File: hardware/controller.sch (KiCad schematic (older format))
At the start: 13 parts, among them U1 STM32F103C8Tx, Y1 16Mhz

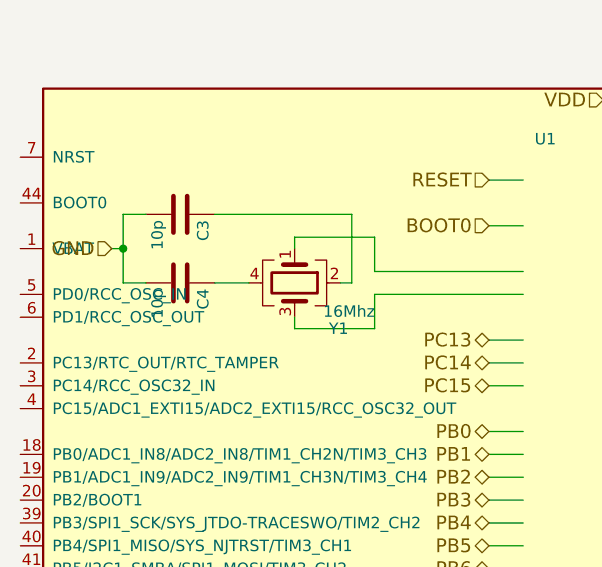
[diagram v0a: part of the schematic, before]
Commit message: stm layout
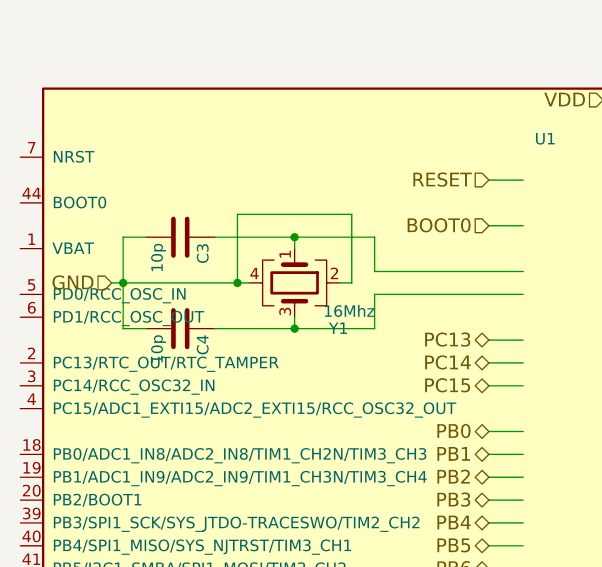
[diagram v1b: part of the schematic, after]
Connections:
- wire segments 106 -> 110
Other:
- moved on the sheet: C3, C4
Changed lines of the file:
@@
 Wire Wire Line
 	4300 3200 4300 3150
-Wire Wire Line
-	4500 3000 4550 3000
-Wire Wire Line
-	4550 3000 4550 2700
-Wire Wire Line
-	4550 2700 3950 2700
 $Comp
 L Device:C C3
 U 1 1 5AE86EDC
-P 3800 2700
-F 0 "C3" H 3825 2800 50  0000 L CNN
-F 1 "10p" H 3825 2600 50  0000 L CNN
-F 2 "_Generic:0603_Small" H 3838 2550 50  0001 C CNN
-F 3 "" H 3800 2700 50  0001 C CNN
-	1    3800 2700
+P 3800 2800
+F 0 "C3" H 3825 2900 50  0000 L CNN
+F 1 "10p" H 3825 2700 50  0000 L CNN
+F 2 "_Generic:0603_Small" H 3838 2650 50  0001 C CNN
+F 3 "" H 3800 2800 50  0001 C CNN
+	1    3800 2800
 	0    1    1    0
 $EndComp
@@
 L Device:C C4
 U 1 1 5AE86F0D
-P 3800 3000
-F 0 "C4" H 3825 3100 50  0000 L CNN
-F 1 "10p" H 3825 2900 50  0000 L CNN
-F 2 "_Generic:0603_Small" H 3838 2850 50  0001 C CNN
-F 3 "" H 3800 3000 50  0001 C CNN
-	1    3800 3000
+P 3800 3200
+F 0 "C4" H 3825 3300 50  0000 L CNN
+F 1 "10p" H 3825 3100 50  0000 L CNN
+F 2 "_Generic:0603_Small" H 3838 3050 50  0001 C CNN
+F 3 "" H 3800 3200 50  0001 C CNN
+	1    3800 3200
 	0    1    1    0
 $EndComp
-Wire Wire Line
-	3950 3000 4100 3000
-Text HLabel 3500 2850 0    60   Input ~ 0
-GND
-Wire Wire Line
-	3500 2850 3550 2850
-Wire Wire Line
-	3550 2700 3550 2850
-Wire Wire Line
-	3550 2700 3650 2700
-Wire Wire Line
-	3550 3000 3650 3000
-Connection ~ 3550 2850
+Text HLabel 3500 3000 0    60   Input ~ 0
+GND
+Wire Wire Line
+	3500 3000 3550 3000
+Wire Wire Line
+	3550 2800 3550 3000
+Wire Wire Line
+	3550 2800 3650 2800
+Wire Wire Line
+	3550 3200 3650 3200
+Connection ~ 3550 3000
 Text HLabel 5150 3250 0    60   BiDi ~ 0
 PC13
@@
 $EndComp
 Wire Wire Line
-	3550 2850 3550 3000
+	3550 3000 3550 3200
 Wire Wire Line
 	5800 5500 5900 5500
@@
 	6200 2200 6200 2350
 Connection ~ 6100 2200
+Wire Wire Line
+	4300 2800 3950 2800
+Connection ~ 4300 2800
+Wire Wire Line
+	3950 3200 4300 3200
+Connection ~ 4300 3200
+Wire Wire Line
+	4100 3000 4050 3000
+Wire Wire Line
+	4050 2700 4050 3000
+Connection ~ 4050 3000
+Wire Wire Line
+	4050 3000 3550 3000
+Wire Wire Line
+	4500 3000 4550 3000
+Wire Wire Line
+	4550 3000 4550 2700
+Wire Wire Line
+	4050 2700 4550 2700
 $EndSCHEMATC
